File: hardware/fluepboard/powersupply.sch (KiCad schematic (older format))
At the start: 17 parts, among them U2 MCP16301

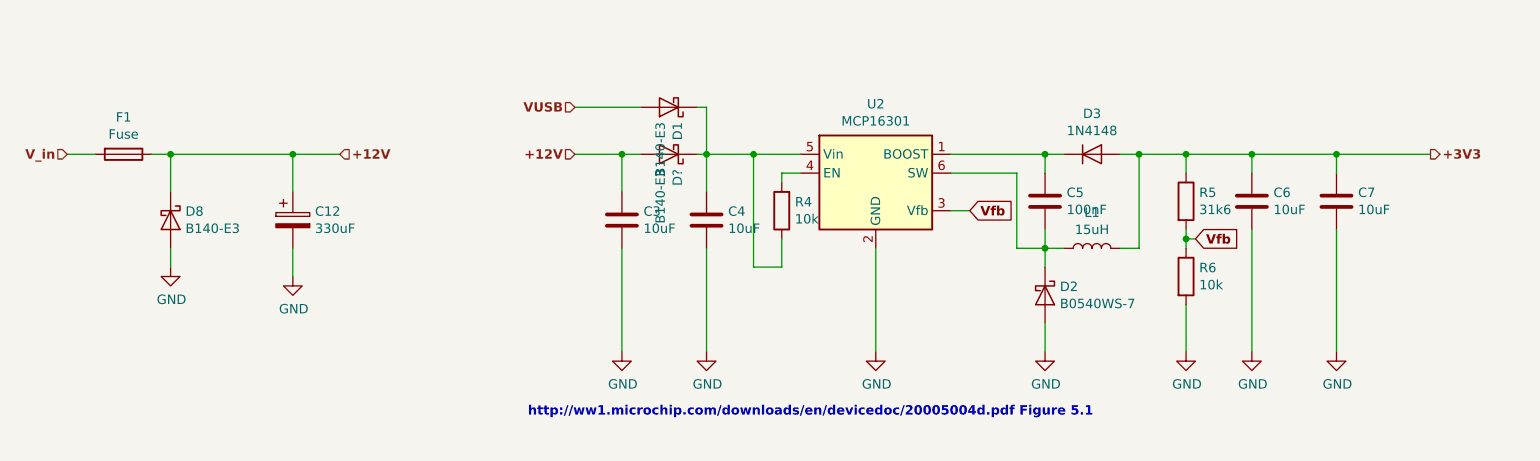
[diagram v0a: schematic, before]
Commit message: Commit jlcpcb compatible version
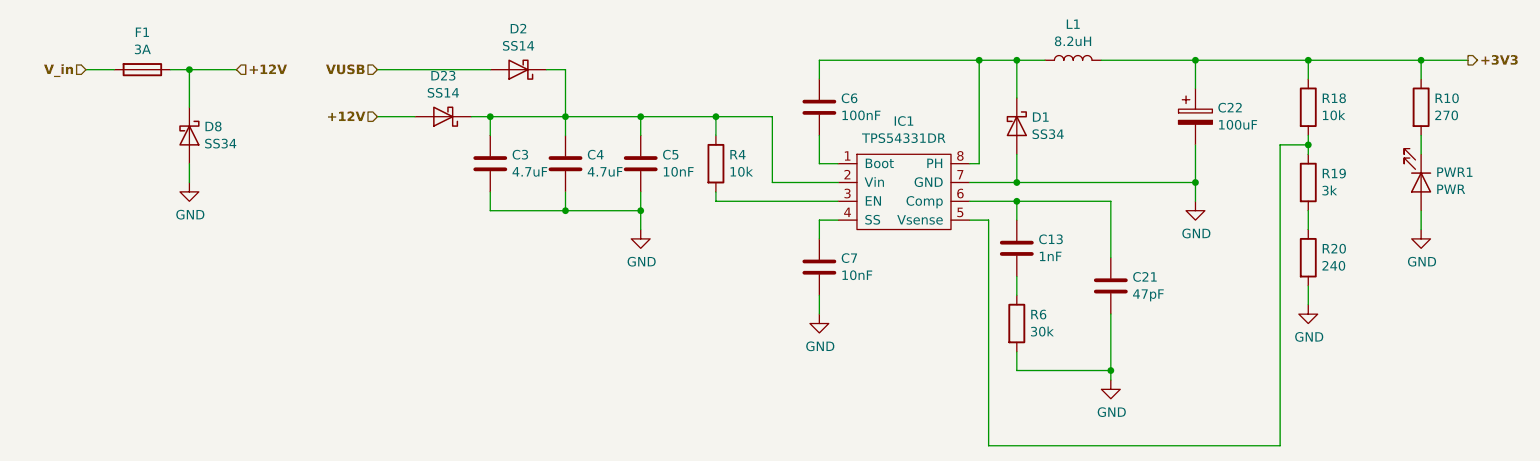
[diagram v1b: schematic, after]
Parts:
- removed C12: 330uF, Capacitor_SMD:CP_Elec_6.3x7.7, symbol Device:CP
- removed D1, D?: B140-E3, Diode_SMD:D_SMA, symbol Diode:B140-E3
- removed D2: B0540WS-7, Diode_SMD:D_SOD-323, symbol Diode:B140-E3
- removed D3: 1N4148, Diode_SMD:D_SOD-323, symbol Diode:1N4148
- removed R5: 31k6, Resistor_SMD:R_0805_2012Metric, symbol Device:R
- removed U2: MCP16301, Package_TO_SOT_SMD:SOT-23-6, symbol Regulator_Switching:MCP16301
- added C13: 1nF, Capacitor_SMD:C_0603_1608Metric, symbol Device:C
- added C21: 47pF, Capacitor_SMD:C_0603_1608Metric, symbol Device:C
- added C22: 100uF, Capacitor_Tantalum_SMD:CP_EIA-3528-21_Kemet-B, symbol Device:CP
- added D1: SS34, Diode_SMD:D_SMA, symbol Diode:B340
- added D2, D23: SS14, Diode_SMD:D_SMA, symbol Device:D_Schottky
- added IC1: TPS54331DR, Package_SO:SOIC-8_3.9x4.9mm_P1.27mm, symbol fluepdot:TPS54331DR
- added PWR1: PWR, Diode_SMD:D_0805_2012Metric, symbol Device:LED
- added R10: 270, Resistor_SMD:R_0603_1608Metric, symbol Device:R
- added R18: 10k, Resistor_SMD:R_0603_1608Metric, symbol Device:R
- added R19: 3k, Resistor_SMD:R_0603_1608Metric, symbol Device:R
- added R20: 240, Resistor_SMD:R_0603_1608Metric, symbol Device:R
- C3, C4: value 10uF -> 4.7uF; Description (none) -> MULTILAYER CERAMIC CAPACITORS MLCC - SMD/SMT 4.7UF 25V 0805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; Extended Part (none) -> 0; LCSC (none) -> C1779; Manufacturer (none) -> CL21A475KAQNNNE; Octopart FEHLER!!! -> (none)
- C5: value 100nF -> 10nF; footprint Capacitor_SMD:C_0805_2012Metric -> Capacitor_SMD:C_0603_1608Metric; Description (none) -> MULTILAYER CERAMIC CAPACITORS MLCC - SMD/SMT 10NF 50V 0603 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; Extended Part (none) -> 0; LCSC (none) -> C57112; Manufacturer (none) -> 0603B103K500NT; Octopart C0805C104Z5VACTU -> (none)
- C6: value 10uF -> 100nF; footprint Capacitor_SMD:C_0805_2012Metric -> Capacitor_SMD:C_0603_1608Metric; Description (none) -> MULTILAYER CERAMIC CAPACITORS MLCC - SMD/SMT 100NF 50V 0603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; Extended Part (none) -> 0; LCSC (none) -> C14663; Manufacturer (none) -> CC0603KRX7R9BB104; Octopart FEHLER!!! -> (none)
- C7: value 10uF -> 10nF; footprint Capacitor_SMD:C_0805_2012Metric -> Capacitor_SMD:C_0603_1608Metric; Description (none) -> MULTILAYER CERAMIC CAPACITORS MLCC - SMD/SMT 10NF 50V 0603 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; Extended Part (none) -> 0; LCSC (none) -> C57112; Manufacturer (none) -> 0603B103K500NT; Octopart FEHLER!!! -> (none)
- D8: value B140-E3 -> SS34; Description (none) -> SCHOTTKY BARRIER DIODES (SBD) SMA(DO-214AC) ROHS; Extended Part (none) -> 0; LCSC (none) -> C84635; Manufacturer (none) -> SS34
- F1: value Fuse -> 3A; Description (none) -> SURFACE MOUNT FUSES 1206 ROHS; Extended Part (none) -> 1; LCSC (none) -> C182441; Manufacturer (none) -> 12D1300C; Octopart SF-1206F400-2 -> (none)
- L1: value 15uH -> 8.2uH; footprint fluepdot:744025150 -> fluepdot:SMD-PIND-6.6x7.1x3.0_1.6x3.0; Description (none) -> POWER INDUCTORS 8.2UH ±20% 5A SMD,6.6X7.1X3.0MM ROHS; Extended Part (none) -> 1; LCSC (none) -> C132140; Manufacturer (none) -> MWSA0603-8R2MT; Octopart 744025150 -> (none)
- R4: footprint Resistor_SMD:R_0805_2012Metric -> Resistor_SMD:R_0603_1608Metric; Description (none) -> CHIP RESISTOR - SURFACE MOUNT 10KOHMS ±1% 1/10W 0603 ROHS; Extended Part (none) -> 0; LCSC (none) -> C25804; Manufacturer (none) -> 0603WAF1002T5E; Octopart RC0805FR-0710KL -> (none)
- R6: value 10k -> 30k; footprint Resistor_SMD:R_0805_2012Metric -> Resistor_SMD:R_0603_1608Metric; Description (none) -> CHIP RESISTOR - SURFACE MOUNT 30KOHMS ±1% 1/10W 0603 ROHS; Extended Part (none) -> 0; LCSC (none) -> C22984; Manufacturer (none) -> 0603WAF1002T5E; Octopart RC0805FR-0710KL -> (none)
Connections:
- net +12V: now also D23.2 (A); no longer C3.1
- net +3V3: now also C22.1, R10.1, R18.1; no longer C6.1, C7.1
- net GND: now also C5.2, C21.2, C22.2, D1.2 (A), IC1.7 (GND), PWR1.2 (A), R20.2; no longer C6.2
- net VUSB: now also D2.2 (A)
- net at C5.1: now also C3.1, C4.1, R4.1, D2.1 (K), D23.1 (K), IC1.2 (Vin)
- net at R4.2: now also IC1.3 (EN)
- net at L1.1: now also C6.1, D1.1 (K), IC1.8 (PH); no longer C5.2
- net Vfb: no longer names the net of R6.1
- net Vfb: now also C13.2
- new net: C6.2, IC1.1 (Boot)
- new net: C7.1, IC1.4 (SS)
- new net: IC1.5 (Vsense), R18.2, R19.1
- new net: C13.1, C21.1, IC1.6 (Comp)
- new net: R19.2, R20.1
- new net: PWR1.1 (K), R10.2
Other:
- note removed: "http://ww1.microchip.com/downloads/en/devicedoc/20005004d.pdf Figure 5.1"
- moved on the sheet: D8, F1
